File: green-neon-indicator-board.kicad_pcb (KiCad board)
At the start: 2 copper layers, 20 x 20 mm, 0 parts

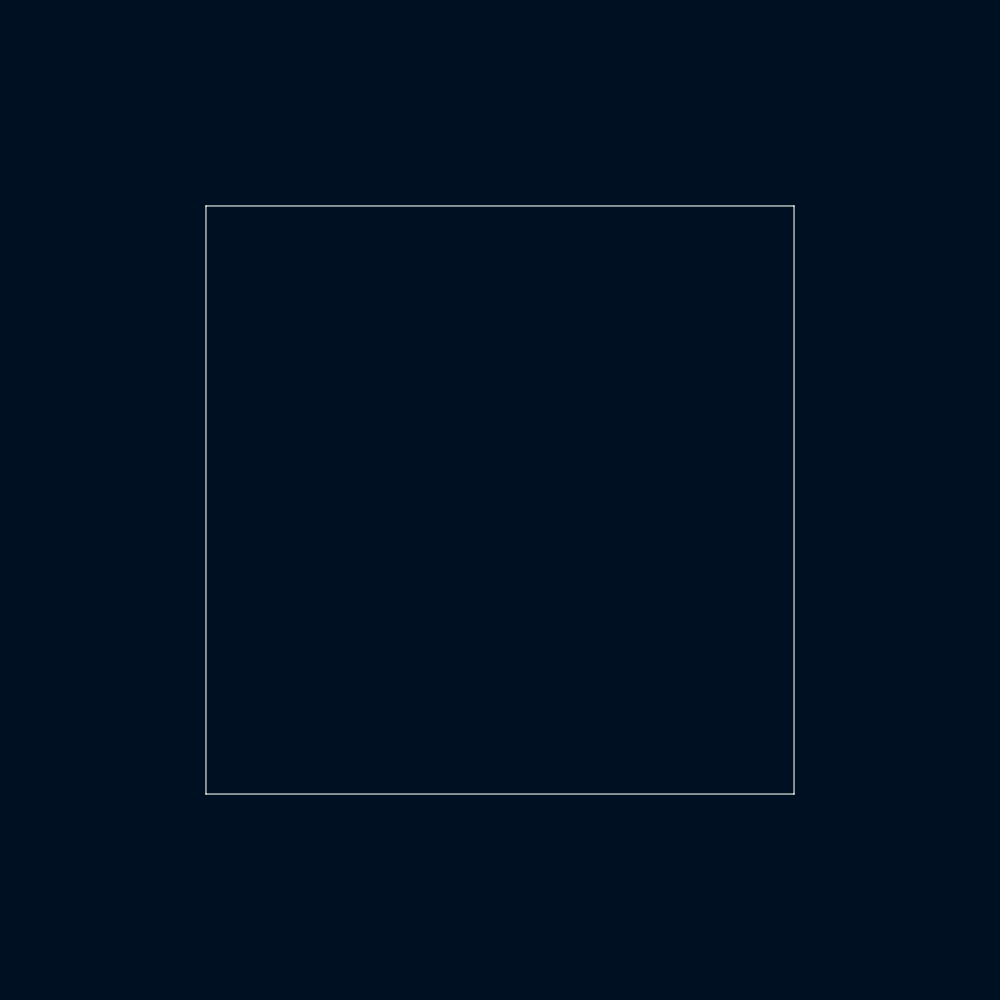
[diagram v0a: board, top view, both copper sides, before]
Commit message: Select all component values, initial layout and routing
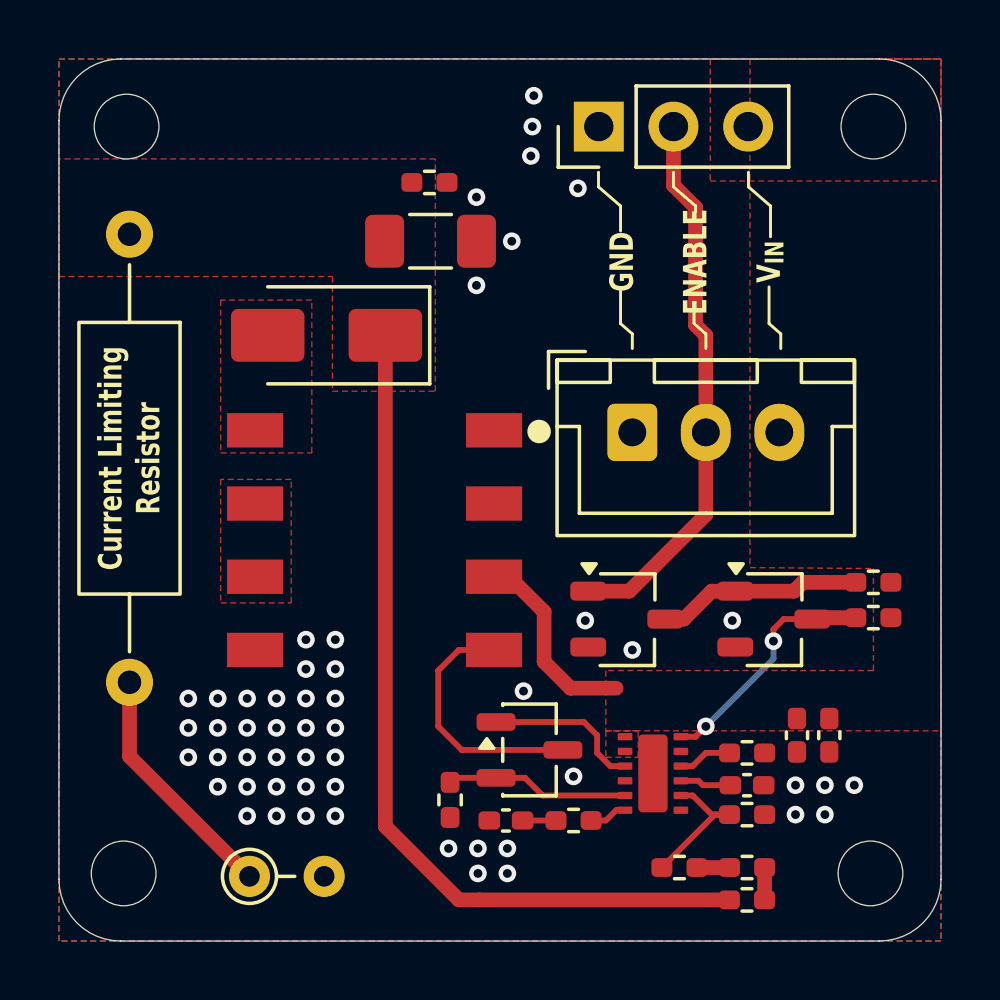
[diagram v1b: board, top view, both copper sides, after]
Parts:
- added C1: 10u, Capacitor_SMD:C_0402_1005Metric_Pad0.74x0.62mm_HandSolder, F.Cu at (111.2, 108.0)
- added C2: 100n, Capacitor_SMD:C_0402_1005Metric_Pad0.74x0.62mm_HandSolder, F.Cu at (110.1, 108.0)
- added C3: 100n, Capacitor_SMD:C_0402_1005Metric_Pad0.74x0.62mm_HandSolder, F.Cu at (108.4, 109.7)
- added C4: 470n, Capacitor_SMD:C_0402_1005Metric_Pad0.74x0.62mm_HandSolder, F.Cu at (100.2, 110.9)
- added C5: 100n, Capacitor_SMD:C_1206_3216Metric_Pad1.33x1.80mm_HandSolder, F.Cu at (97.6, 91.2)
- added D1: US1G-E3/61T, Diode_SMD:D_SMA, F.Cu at (94.1, 94.4)
- added J1: 1x3 THT Headers, Connector_PinHeader_2.54mm:PinHeader_1x03_P2.54mm_Vertical, F.Cu at (103.4, 87.3)
- added J2: JST XH Compatible, Connector_JST:JST_XH_B3B-XH-A_1x03_P2.50mm_Vertical, F.Cu at (104.5, 97.7)
- added NE1: Green Neon Lamp, Resistor_THT:R_Axial_DIN0204_L3.6mm_D1.6mm_P2.54mm_Vertical, F.Cu at (91.5, 112.8)
- added Q1: IRLML0100TRPBF, Package_TO_SOT_SMD:SOT-23-3, F.Cu at (101.0, 108.5)
- added Q2: PJA138K, Package_TO_SOT_SMD:TSOT-23, F.Cu at (109.3, 104.0)
- added Q3: PJA138K, Package_TO_SOT_SMD:TSOT-23, F.Cu at (104.3, 104.0)
- added R10: 1M, Resistor_SMD:R_0402_1005Metric_Pad0.72x0.64mm_HandSolder, F.Cu at (97.6, 89.2)
- added R11: 330k, Resistor_THT:R_Axial_DIN0309_L9.0mm_D3.2mm_P15.24mm_Horizontal, F.Cu at (87.4, 91.0)
- added R12: 10k, Resistor_SMD:R_0402_1005Metric_Pad0.72x0.64mm_HandSolder, F.Cu at (112.7, 102.8)
- added R13: 100k, Resistor_SMD:R_0402_1005Metric_Pad0.72x0.64mm_HandSolder, F.Cu at (112.7, 104.0)
- added R3: 110k, Resistor_SMD:R_0402_1005Metric_Pad0.72x0.64mm_HandSolder, F.Cu at (108.4, 108.6)
- added R4: 10k, Resistor_SMD:R_0402_1005Metric_Pad0.72x0.64mm_HandSolder, F.Cu at (102.5, 110.9)
- added R5: 0.5, Resistor_SMD:R_0402_1005Metric_Pad0.72x0.64mm_HandSolder, F.Cu at (98.3, 110.2)
- added R6: 499k, Resistor_SMD:R_0402_1005Metric_Pad0.72x0.64mm_HandSolder, F.Cu at (108.4, 113.6)
- added R7: 499k, Resistor_SMD:R_0402_1005Metric_Pad0.72x0.64mm_HandSolder, F.Cu at (108.4, 112.5)
- added R8: 499k, Resistor_SMD:R_0402_1005Metric_Pad0.72x0.64mm_HandSolder, F.Cu at (106.1, 112.5)
- added R9: 10k, Resistor_SMD:R_0402_1005Metric_Pad0.72x0.64mm_HandSolder, F.Cu at (108.4, 110.7)
- added REF**: MountingHole_2.2mm_M2_DIN965, MountingHole:MountingHole_2.2mm_M2_DIN965, F.Cu at (112.7, 87.3)
- added REF**: MountingHole_2.2mm_M2_DIN965, MountingHole:MountingHole_2.2mm_M2_DIN965, F.Cu at (112.6, 112.7)
- added REF**: MountingHole_2.2mm_M2_DIN965, MountingHole:MountingHole_2.2mm_M2_DIN965, F.Cu at (87.2, 112.7)
- added REF**: MountingHole_2.2mm_M2_DIN965, MountingHole:MountingHole_2.2mm_M2_DIN965, F.Cu at (87.3, 87.3)
- added T1: WURTH_750311692, CustomLibraries:WURTH_750311692, F.Cu at (95.7, 101.4)
- added U1: ~, CustomLibraries:LM5155, F.Cu at (105.2, 109.3)
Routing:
- net +150V: track 0.00 -> 29.4 mm
- net /EN_INPUT: track 0.00 -> 18.7 mm
- net Net-(Q1-D): track 0.00 -> 8.66 mm
- net Net-(NE1-Pad1): track 0.00 -> 8.29 mm
- net /BOOST_EN: track 0.00 -> 8.21 mm, vias 0 -> 2
- net Net-(Q2-G): track 0.00 -> 7.00 mm
- net V_{BIAS}: track 0.00 -> 6.72 mm
- net Net-(Q1-S): track 0.00 -> 6.26 mm
- net Net-(Q1-G): track 0.00 -> 5.36 mm
- net Net-(U1-FB): track 0.00 -> 4.97 mm
- net Net-(U1-RT): track 0.00 -> 1.84 mm
- net Net-(U1-SS): track 0.00 -> 1.74 mm
- net Net-(U1-COMP): track 0.00 -> 1.30 mm
- net Net-(C4-Pad1): track 0.00 -> 1.14 mm
- net Net-(R7-Pad2): track 0.00 -> 1.11 mm
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- added copper zone on F.Cu, net +150V
- added copper zone on B.Cu, net GND
- added copper zone on F.Cu, net GND
- added copper zone on F.Cu, net Net-(D1-A)
- added copper zone on F.Cu, net Net-(T1-SB)
- added copper zone on F.Cu, net V_{BIAS}
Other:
- board size 20 x 20 mm -> 30 x 30 mm
- board text added: "Current Limiting Resistor"
- board text added: "ENABLE"
- board text added: "GND"
- board text added: "V_{IN}"
